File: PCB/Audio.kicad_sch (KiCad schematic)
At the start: 50 parts, among them J3 AUDIO JACK, Q1 IRLML2502, Q2 IRLML2502, Q3 IRLML2502, Q4 IRLML2502, Q5 IRLML2502, Q6 IRLML2502, U20 xc7z020clg484, U9 TLV320AIC3104

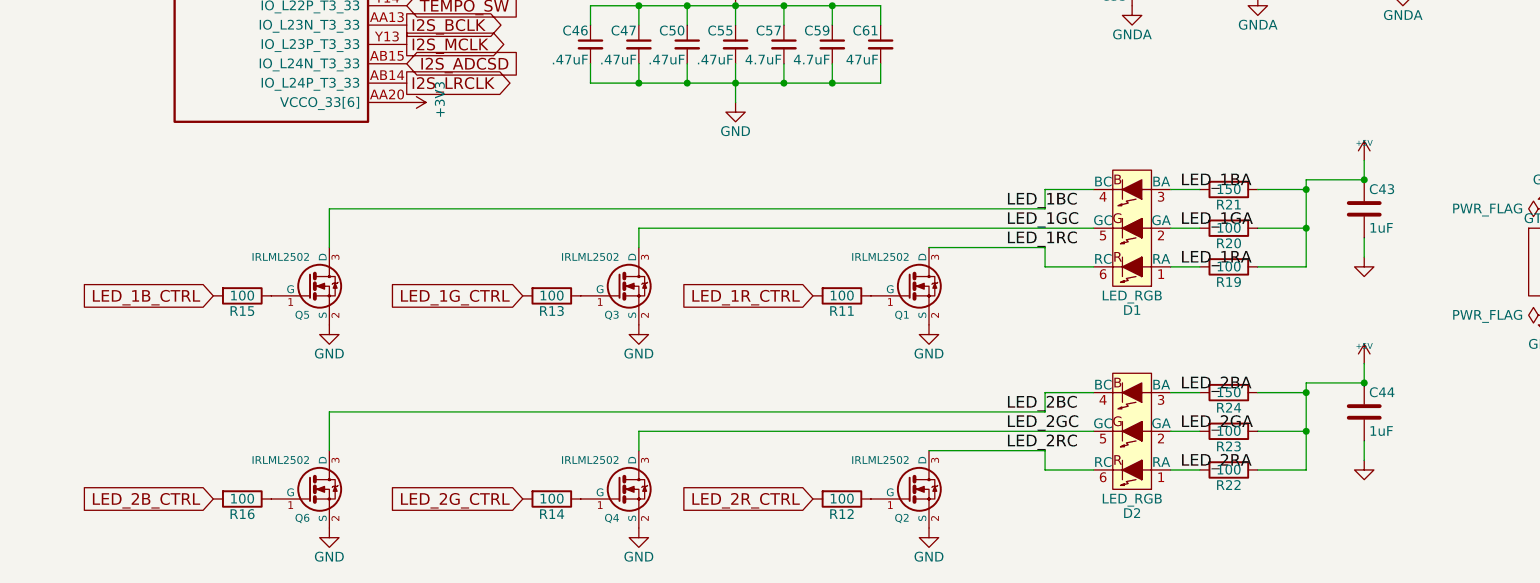
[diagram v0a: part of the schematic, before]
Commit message: [+] add xdc files
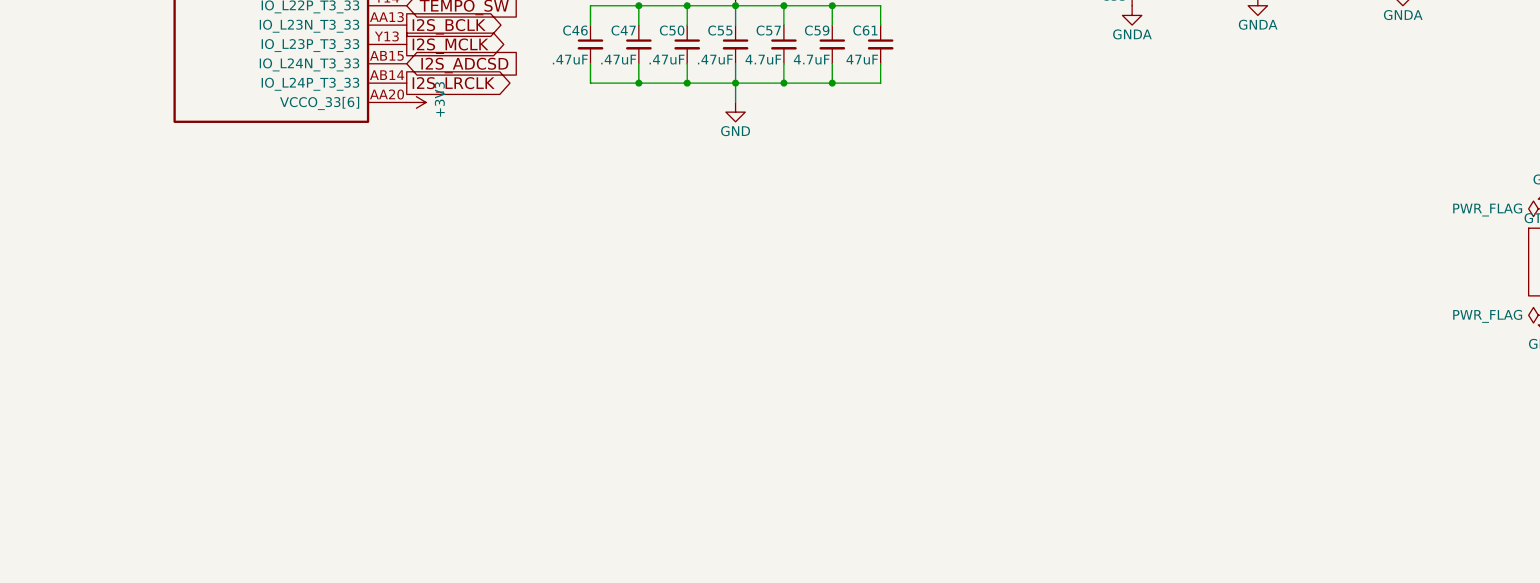
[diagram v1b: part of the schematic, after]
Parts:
- removed C43, C44: 1uF, Capacitor_SMD:C_0402_1005Metric, symbol Device:C
- removed D1, D2: LED_RGB, DFTcustom:PLCC6-SM-RGB-LED, symbol DFTBoard-rescue:LED_RGB-RESCUE-DFTBoard-
- removed Q1, Q2, Q3, Q4, Q5, Q6: IRLML2502, Package_TO_SOT_SMD:SOT-23, symbol DFTBoard-rescue:IRLML2502-
- removed R11, R12, R13, R14, R15, R16, R19, R20, R22, R23: 100, Resistor_SMD:R_0402_1005Metric, symbol Device:R
- removed R21, R24: 150, Resistor_SMD:R_0402_1005Metric, symbol Device:R
